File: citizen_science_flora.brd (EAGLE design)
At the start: 86.6 x 79.6 mm, 118 parts, among them IC1 W25Q64JVXGIQ, J1 SM03B-SRSS-TB(LF)(SN), J2 TYPE-C-31-M-12, J4 60312202114511, J5 60312202114511, J6 TSM-102-02-S-SH, Q1 220mA/50V/3.5Ω, Q2 BSS138, U1 RP2350A, U10 PCF8563T/F4,118, U11 OPS-S56AAF5, U12 OPS-S56AAF5, U13 OPS-S56AAF5, U14 OPS-S56AAF5, U15 SN74LVC1T45DBVRG4, U2 APS6404L-3SQR-ZR, U3 ESP32-C3-MINI-1-N4, U4 MIC5504-3.3YM5-T5, U5 BME690, U6 ADM3260ARSZ, U7 ENS210-LQFM, U8 SFH6325-X017TEL0631, U9 AS3935-BQFT, Y1 12MHz

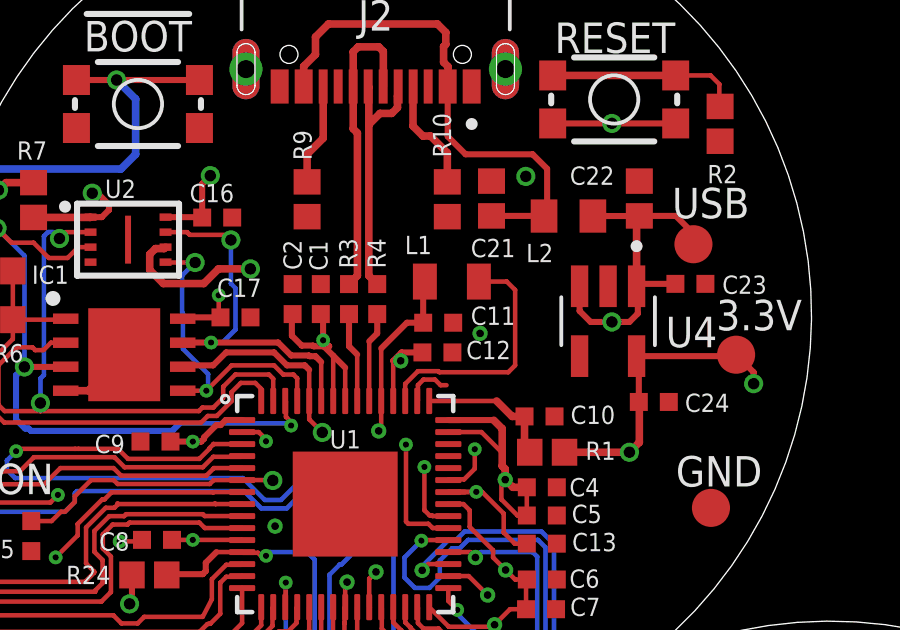
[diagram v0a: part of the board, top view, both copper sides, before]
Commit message: updated gerber files
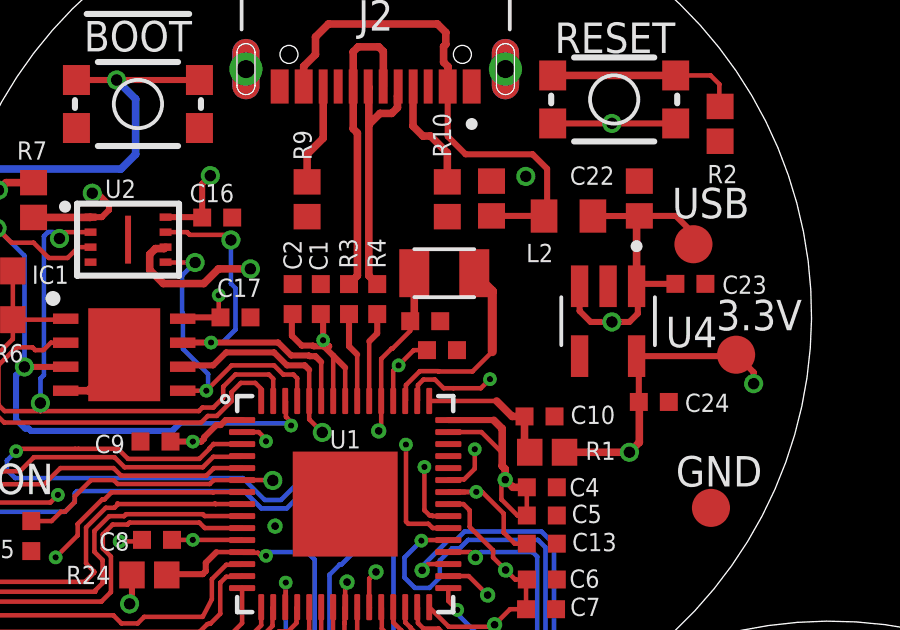
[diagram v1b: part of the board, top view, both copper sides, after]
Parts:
- removed L1: 3.3µH, SparkFun-Coils:0805
- added L4: 3.3uH, LQH2MCN120K02L:IND_LQH2MCN120K02L
- moved C11 0.43 mm to (15.4, 25.1)
- moved C12 0.17 mm to (15.9, 24.2)
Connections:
- net 1.1V: now also L4.2; no longer L1.2
- net N$2: now also L4.1; no longer L1.1
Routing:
- net GND: track 22.1 -> 23.7 mm
- net N$2: track 8.36 -> 6.75 mm
- net 3.3V: track 151.8 -> 150.8 mm
